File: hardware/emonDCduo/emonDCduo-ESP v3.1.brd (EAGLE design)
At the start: 99.1 x 76.5 mm, 73 parts, among them J5 455-1750-1-ND, P1 B4B-PH-K, Y1 32Khz

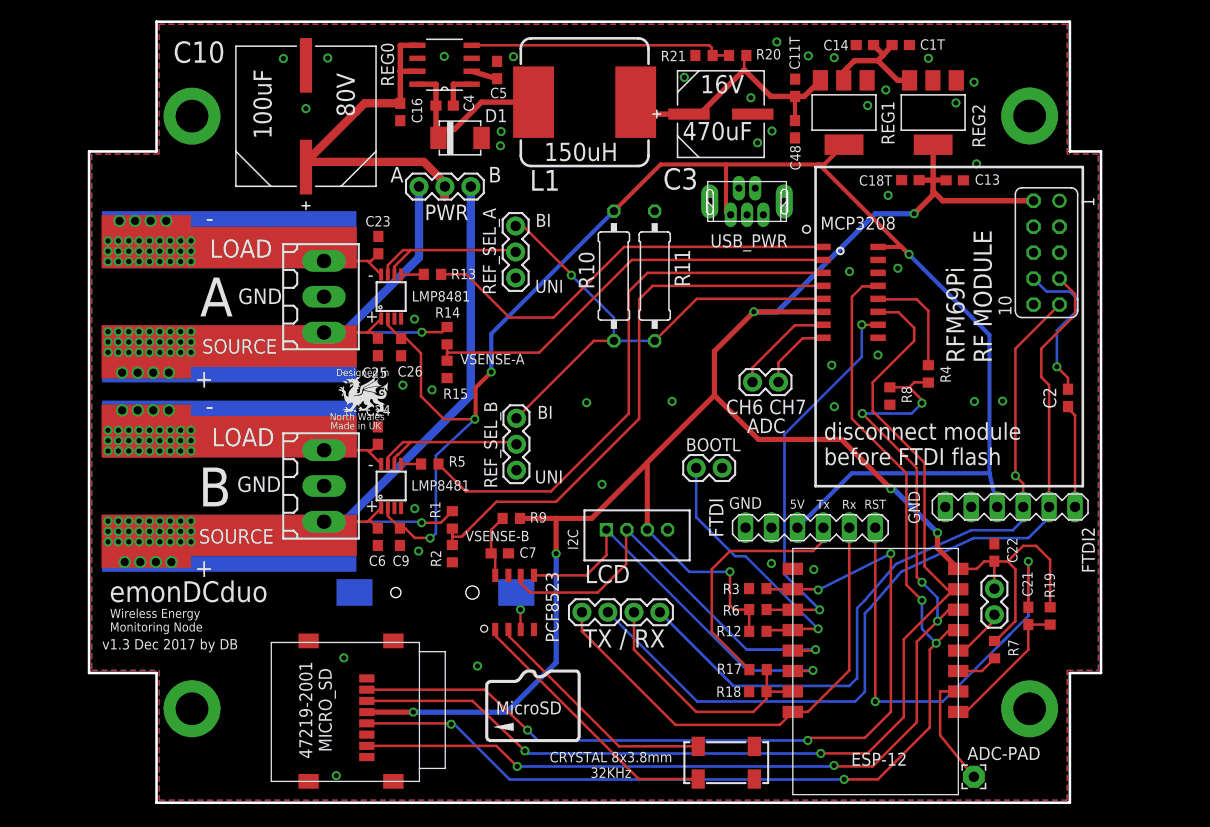
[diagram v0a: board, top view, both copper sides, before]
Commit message: commit v3.1
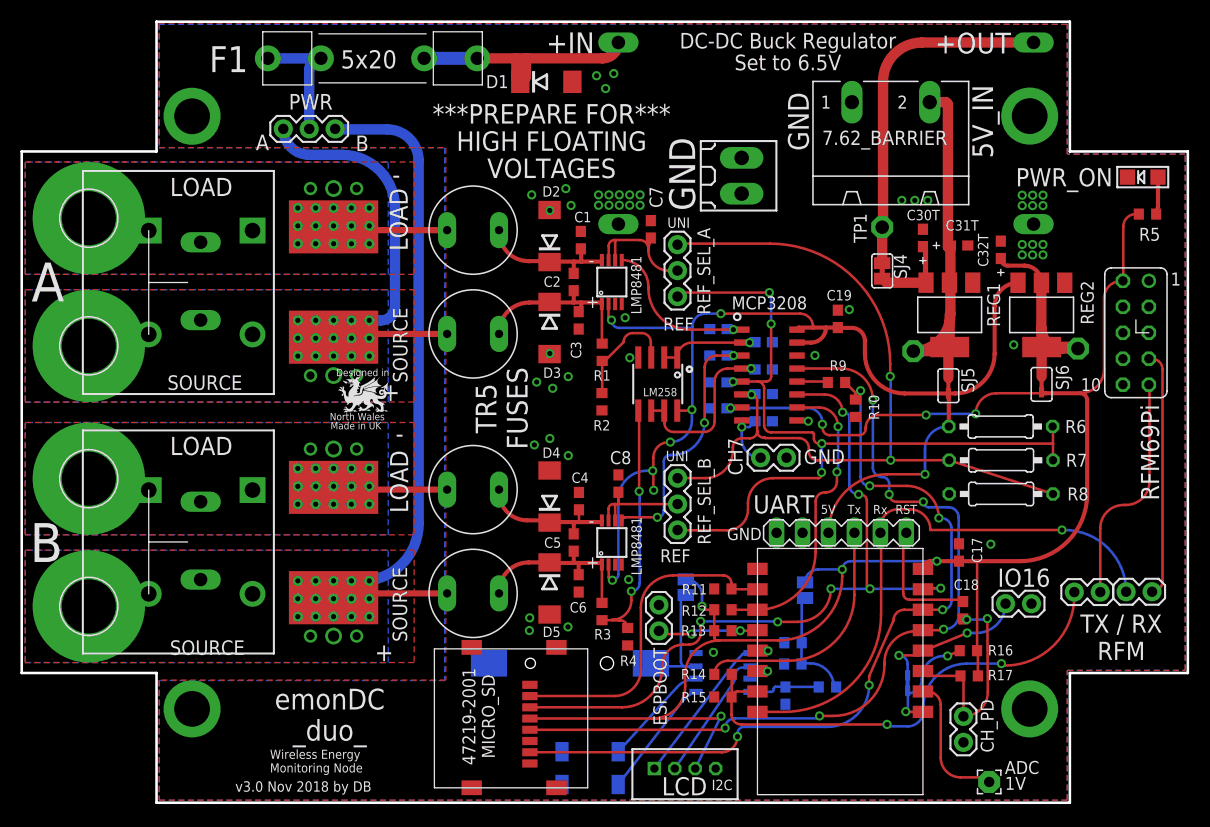
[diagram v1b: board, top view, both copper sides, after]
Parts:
- removed ADC-PAD: (no value), wirepad:2,15/1,0
- removed BOOTL, IO1: (no value), SparkFun:1X02
- removed C11T, C18T, C1T: 10uF TANT, rcl:C0603
- removed C21, C22, C26: 100nF, rcl:C0603
- removed C23, C24, C25: 0.1uF 100V, rcl:C0603
- removed C48: 0.1uF MLCC, rcl:C0603
- removed FTDI1, FTDI2: FTDI, JeeLabs:MA06-1
- removed L1: SRR1208, inductor-bourns:SSR1208
- removed R18, R19: 10K, rcl:R0603
- removed REG0: MAX5035, MAX5035:21-0111D_SBE-14
- removed SCREW1, SCREW2: (no value), con-weidmueller-sl35:180-3
- removed SCREW_TERM_1, SCREW_TERM_2: EBW_SERIES_15.2MM, EBW series shunt:EBW_SERIES_15.2MM
- removed U$4: 47219-2001_MICROSD, MOLEX 47219-2001:47219-2001_MICROSD
- removed USB_PWR: 5000751517_SD, 5000751517_sd:5000751517_SD
- added 3.3V_BAT, SJ4: (no value), jumper-con:SJ-CON
- added 7.62_BARRIER: GMSTBA2, con-phoenix-762:GMSTBA2
- added ADC: (no value), wirepad:2,15/1,0
- added C1, C8: 0.1uF 100V, rcl:C0603
- added C11, C12, C15: 1nF, rcl:C0603
- added C17, C18, C19: 0.1uF, rcl:C0603
- added C30T, C31T, C32T, C33T: 10uF TANT, rcl7:C0603POL
- added CH_PD, ESPBOOT: (no value), SparkFun:1X02
- added D2, D3, D4, D5: P6SMB75A, diode:DO214AA
- added EBW_A, EBW_B: EBW_SERIES_15.2MM, EBW series SHUNT:EBW_SERIES_15.2MM
- added F1: 445/030_SERIES, LITTELFUSE 455:030 SERIES:445/030_SERIES_LITTELFUSE
- added F2, F3, F4, F5: (no value), fuse:TR5
- added GND: (no value), con-weidmueller-sl35_db:180-2
- added IO16: FACTORY_RESET, SparkFun:1X02
- added LED1: PWR_ON, microbuilder:CHIPLED_1206
- added LM258: (no value), microbuilder:SOIC8_150MIL
- added MH1, MH2, MH3, MH4: 5.3mm, holes-db:5,3//11-PAD
- added MICRO_SD: 47219-2001_MICROSD, MOLEX 47219-2001:47219-2001_MICROSD
- added MOUNT_10.16_A, MOUNT_10.16_B: MOLEX_39970-003, 10.16mm terminal block:2/10,16
- added R16: 10K, rcl:R0603
- added R22: 1K, rcl@1:R0603
- added SJ1, SJ5, SJ6: (no value), jumper-con_db:SJ-CON
- added SJ2: (no value), jumper:SJ
- added TP1, TP2, TP3: TPPAD1-13, testpad:P1-13
- added TP10, TP11, TP4, TP5, TP6, TP7, TP8, TP9: TPPAD1-13Y, testpad:P1-13Y
- added U$2, U$3: (no value), ALIGNMENT_STOP:ALIGNMENT_STOP
- added UART: UART, JeeLabs:MA06-1
- C10: value 100uF 80V (LOW-ESR) -> 1nF; device Panasonic-EEE-EEV-EEF-ECQ:CAPAE1350X1400N -> rcl:C0603
- C13, C14: value 0.1uF -> 1nF
- C16: value 0.1uF 100V -> 1nF
- C2: value 100nF -> 0.1uF 100V
- C3: value 470uF 16V -> 0.1uF 100V; device Panasonic-EEEFK_EEEFP:CAPAE830X1050N -> rcl:C0603
- C4, C5: value 0.1uF 16V MLCC -> 0.1uF 100V
- C7: value 10uF -> 0.1uF 100V
- C9: value 100nF -> 1nF
- D1: value MBRS1100T3G -> P6SMB75A; device diodes:SMB_1 -> diode:DO214AA
- GPIO_1: device con-lsta:FE05-2 -> con-lsta-RFM69Pi:FE05-2_RFM69PI_OULTINE
- J5: value 455-1750-1-ND -> (none)
- P1: device jst-ph:B4B-PH-K -> JST-PH:B4B-PH-K
- PCF8523: device IotaWatt_parts:SOIC_8 -> emonDC parts:SOIC_8
- R1: value 100K 75V -> 1M 100V
- R10: value 10K -> 2K; device rcl:0309/12 -> rcl:R0603
- R11: value 3.16K -> 10K; device rcl:0309/12 -> rcl:R0603
- R13: value 1K -> 10K
- R14: value 100K 75V -> 1k
- R15: value 5.6K -> 2k
- R17: value 5.6K -> 10K
- R2: value 5.6K -> 56K
- R20: value 57.6k -> 10K
- R21: value 13.3k -> 10K
- R3: value 10K -> 1M 100V
- R4: value 1K -> 56K
- R5: value 1K -> 174R
- R6: value 10K -> 10k; device rcl:R0603 -> rcl7:0207/10
- R7: value 10K -> 5.6k; device rcl:R0603 -> rcl7:0207/10
- R8: value 2K -> 174R; device rcl:R0603 -> rcl7:0207/10
- REG1, REG2: device burr-brown:SOT223 -> burr-brown-db:SOT223
- moved R5 74.4 mm to (103.9, 59.4), turned to 180 degrees
- moved R21 60.2 mm to (69.1, 15.4), flipped to the bottom
- moved LOGO1 59.5 mm to (81.6, 2.56)
- moved R20 57.7 mm to (69.2, 17.4), flipped to the bottom
- moved TX 53.3 mm to (101.8, 22.4)
- moved C10 50.0 mm to (66.3, 46.9), flipped to the bottom, turned to 180 degrees
- moved C2 49.7 mm to (47.7, 52.8)
- moved C5 46.9 mm to (47.7, 27.2), turned to 270 degrees
- moved C16 46.7 mm to (66.3, 39.1), flipped to the bottom, turned to 180 degrees
- moved R13 45.0 mm to (62.3, 18.6), turned to 180 degrees
- moved RX 43.2 mm to (99.2, 22.4)
- moved R14 42.8 mm to (62.3, 14.3), turned to 0 degrees
- moved R15 41.9 mm to (62.3, 12.1), turned to 180 degrees
- moved C4 40.9 mm to (48.2, 31.3), turned to 90 degrees
- moved R4 39.1 mm to (53.0, 18.0)
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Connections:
- removed net 3.3V: C13.1, C18T.1, C22.2, ESP-12.16, GPIO_1.2, IO1.2, MCP3208.6, P1.3, R12.2, R19.2, R6.2, R7.2, R9.2, REG2.2, REG2.4, U$4.PIN4
- removed net 5.0V: C14.1, C1T.1, C26.1, C9.1, FTDI1.4, FTDI2.4, MCP3208.16, R10.2, REG1.2, REG1.4, REG2.3, SHUNTMON-A.2, SHUNTMON-B.2, USB_PWR.VBUS
- removed net ADCSHUNT-A: MCP3208.1, R13.2
- removed net ADCSHUNT-B: MCP3208.3, R5.2
- removed net BST: C4.1, REG0.1
- removed net CH6: J5.2, MCP3208.7
- removed net FB: R20.1, R21.2, REG0.4
- removed net LX: C4.2, D1.C, L1.1, REG0.8
- removed net N$10: C7.1, PCF8523.8, R9.1
- removed net N$20: FTDI2.5
- removed net N$30: C21.2, FTDI1.1
- removed net N$301: C2.2, FTDI2.1
- removed net N$4: R13.1, SHUNTMON-A.5
- removed net N$43: CR1220.P+, PCF8523.3
- removed net N$6: R5.1, SHUNTMON-B.5
- removed net REF_INPUT: MCP3208.5, R10.1, R11.2, REF_SEL_A.3, REF_SEL_B.3
- removed net RESTESP: C21.1, ESP-12.9, R19.1
- removed net VD: C5.1, REG0.2
- removed net VSENSEA: MCP3208.2, R14.1, R15.2
- removed net VSENSEB: MCP3208.4, R1.1, R2.2
- removed net V_IN: C10.1, C16.1, PWR.2, REG0.5, REG0.7
- new net +3V3: 3.3V_BAT.1, C15.1, C17.2, ESP-12.16, GPIO_1.2, MCP3208.7, MICRO_SD.PIN4, P1.3, R12.2, R13.2, R16.2, R17.2, R5.2, SJ2.1, SJ6.2
- new net +5V: C19.1, LM258.8, MCP3208.15, MCP3208.16, R6.2, REG2.3, SHUNTMON-A.2, SHUNTMON-B.2, SJ5.2, UART.4
- new net 3.3V_PRE: C32T.1, REG2.2, REG2.4, SJ6.1, TP3.TP
- new net 5V_PRE: 7.62_BARRIER.2, C31T.1, REG1.2, REG1.4, SJ5.1, TP2.TP
- new net ADCSHUNT_A: C9.1, MCP3208.1, SHUNTMON-A.5
- new net ADCSHUNT_B: C11.1, MCP3208.3, SHUNTMON-B.5
- new net BI_REF: C13.1, MCP3208.5, R6.1, R7.2, REF_SEL_A.3, REF_SEL_B.3
- new net LOAD-NEG-A_T: C1.1, C2.1, D2.C, F2.2, SHUNTMON-A.8
- new net LOAD-NEG-B_T: C4.1, C5.1, D4.C, F4.2, SHUNTMON-B.8
- new net N$1: SJ4.1, TP1.TP, TP5.TP
- new net N$5: LED1.A, R5.1
- new net RESET: C18.2, UART.1
- new net RST: ESP-12.9, R16.1, SJ1.1
- new net SOURCE-POS-A_T: C2.2, C3.1, D3.C, F3.2, R1.2, SHUNTMON-A.1
- new net SOURCE-POS-B_T: C5.2, C6.1, D5.C, F5.2, R3.2, SHUNTMON-B.1
- new net UNI_REF: C14.1, MCP3208.6, R7.1, R8.2, REF_SEL_A.1, REF_SEL_B.1
- new net VBAT: 3.3V_BAT.2, CR1220.P+, PCF8523.3
- new net VDD_PCF: C33T.1, PCF8523.8, R22.1
- new net VDD_RTC_POSTJUMPER: R20.1, R21.1, R22.2, SJ2.2
- new net VSENSE_A: LM258.3, R1.1, R2.2
- new net VSENSE_A_BUFF: C10.1, LM258.1, LM258.2, MCP3208.2
- new net VSENSE_B: LM258.5, R3.1, R4.2
- new net VSENSE_B_BUFF: C12.1, LM258.6, LM258.7, MCP3208.4
- new net V_IN_POSTFUSE: D1.C, F1.P$3, F1.P$4, TP4.TP
- new net V_IN_PREFUSE: F1.P$1, F1.P$2, PWR.2
- net 6.5V: now also C30T.1, SJ4.2; no longer C11T.1, C3.1, C48.1, L1.2, R20.2
- net ADC: now also ADC.1; no longer ADC-PAD.1
- net CH7: now also C16.1
- net CH_PD: now also C18.1, CH_PD.1, R17.1; no longer R7.1
- net D0/RX: no longer FTDI2.2
- net D1/TX: no longer FTDI2.3
- net ESPRX: now also R14.2, R15.1; no longer R17.2, R18.1
- net ESPTX: now also UART.2; no longer FTDI1.2
- net GND: now also 7.62_BARRIER.1, C1.2, C17.1, C19.2, C30T.2, C31T.2, C32T.2, C33T.2, C4.2, C8.2, CH_PD.2, D2.A, D3.A, D4.A, D5.A, ESPBOOT.1, GND.1, GND.2, IO16.2, J5.2, LED1.C, LM258.4, MICRO_SD.P$1, MICRO_SD.P$2, MICRO_SD.P$3, MICRO_SD.P$4, MICRO_SD.PIN6, R10.2, R11.2, R15.2, R4.1, TP6.TP, TP7.TP, UART.6; no longer BOOTL.1, C10.2, C11T.2, C13.2, C14.2, C16.2, C18T.2, C1T.2, C22.1, C23.1, C24.1, C25.2, C26.2, C48.2, C5.2, C9.2, FTDI1.6, FTDI2.6, MCP3208.15, R11.1, R15.1, R18.2, R21.1, R3.2, REF_SEL_A.1, REF_SEL_B.1, REG0.3, REG0.6, SCREW1.2, SCREW2.2, U$4.P$1, U$4.P$2, U$4.P$3, U$4.P$4, U$4.PIN6, USB_PWR.GND1, USB_PWR.GND2, USB_PWR.GND3
- net GPIO0: now also ESPBOOT.2, R13.1; no longer BOOTL.2, R12.1
- net GPIO12: now also MICRO_SD.PIN7, R10.1, R9.2; no longer R4.1, R8.2, U$4.PIN7
- net GPIO12A: now also R9.1; no longer R4.2
- net GPIO13: now also MICRO_SD.PIN3; no longer U$4.PIN3
- net GPIO14: now also MICRO_SD.PIN5; no longer U$4.PIN5
- net GPIO15: now also MICRO_SD.PIN2, R11.1; no longer R3.1, U$4.PIN2
- net GPIO16: now also IO16.1, SJ1.2; no longer IO1.1
- net GPIO2: now also R12.1; no longer R6.1
- net LOAD-NEG-A: now also EBW_B.P$18, EBW_B.P$19, EBW_B.P$2, EBW_B.P$20, EBW_B.P$21, EBW_B.P$22, EBW_B.P$23, EBW_B.P$24, EBW_B.P$25, EBW_B.P$26, EBW_B.P$27, EBW_B.P$28, EBW_B.P$29, EBW_B.P$30, EBW_B.P$31, EBW_B.P$32, EBW_B.P$36, EBW_B.P$37, EBW_B.P$38, F2.1, MH2.B5,5, MOUNT_10.16_A.P$1, MOUNT_10.16_A.P$2, TP11.TP; no longer C23.2, SCREW1.1, SCREW_TERM_1.P$2, SHUNTMON-A.8
- net LOAD-NEG-B: now also EBW_A.P$18, EBW_A.P$19, EBW_A.P$2, EBW_A.P$20, EBW_A.P$21, EBW_A.P$22, EBW_A.P$23, EBW_A.P$24, EBW_A.P$25, EBW_A.P$26, EBW_A.P$27, EBW_A.P$28, EBW_A.P$29, EBW_A.P$30, EBW_A.P$31, EBW_A.P$32, EBW_A.P$36, EBW_A.P$37, EBW_A.P$38, F4.1, MH4.B5,5, MOUNT_10.16_B.P$1, MOUNT_10.16_B.P$2, TP9.TP; no longer C24.2, SCREW2.1, SCREW_TERM_2.P$2, SHUNTMON-B.8
- net N$32: now also MICRO_SD.PIN8; no longer U$4.PIN8
- net N$36: now also R14.1, UART.3; no longer FTDI1.3, R17.1
- net N$7: now also MICRO_SD.PIN1; no longer U$4.PIN1
- net REF_A_INPUT: now also C7.1
- net REF_B_INPUT: now also C8.1
- net SCL: now also ESP-12.6; no longer ESP-12.5
- net SDA: now also ESP-12.5; no longer ESP-12.6
- net SOURCE-POS-A: now also EBW_B.P$1, EBW_B.P$10, EBW_B.P$11, EBW_B.P$12, EBW_B.P$13, EBW_B.P$14, EBW_B.P$15, EBW_B.P$16, EBW_B.P$17, EBW_B.P$3, EBW_B.P$33, EBW_B.P$34, EBW_B.P$35, EBW_B.P$4, EBW_B.P$5, EBW_B.P$6, EBW_B.P$7, EBW_B.P$8, EBW_B.P$9, F3.1, MH1.B5,5, MOUNT_10.16_A.P$3, MOUNT_10.16_A.P$4, TP10.TP; no longer C25.1, R14.2, SCREW1.3, SCREW_TERM_1.P$1, SHUNTMON-A.1
- net SOURCE-POS-B: now also EBW_A.P$1, EBW_A.P$10, EBW_A.P$11, EBW_A.P$12, EBW_A.P$13, EBW_A.P$14, EBW_A.P$15, EBW_A.P$16, EBW_A.P$17, EBW_A.P$3, EBW_A.P$33, EBW_A.P$34, EBW_A.P$35, EBW_A.P$4, EBW_A.P$5, EBW_A.P$6, EBW_A.P$7, EBW_A.P$8, EBW_A.P$9, F5.1, MH3.B5,5, MOUNT_10.16_B.P$3, MOUNT_10.16_B.P$4, TP8.TP; no longer C6.1, R1.2, SCREW2.3, SCREW_TERM_2.P$1, SHUNTMON-B.1
- net _RESET: no longer C2.1
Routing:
- net 3.3V: track 198.0 -> 0.00 mm, vias 7 -> 0
- net +3V3: track 0.00 -> 172.3 mm, vias 0 -> 8
- net 5.0V: track 171.2 -> 0.00 mm, vias 4 -> 0
- net +5V: track 0.00 -> 113.2 mm, vias 0 -> 8
- net UNI_REF: track 0.00 -> 81.1 mm, vias 0 -> 3
- net BI_REF: track 0.00 -> 79.0 mm, vias 0 -> 5
- net D0/RX: track 84.0 -> 24.0 mm
- net VSENSEB: track 55.7 -> 0.00 mm
- net ADCSHUNT-B: track 54.6 -> 0.00 mm
- net 5V_PRE: track 0.00 -> 53.8 mm
- net GPIO15: track 83.0 -> 31.6 mm, vias 4 -> 0
- net REF_INPUT: track 50.5 -> 0.00 mm, vias 1 -> 0
- net D1/TX: track 72.0 -> 22.5 mm, vias 1 -> 0
- net N$30: track 47.1 -> 0.00 mm, vias 2 -> 0
- net VSENSEA: track 42.3 -> 0.00 mm
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- added copper zone on layer 1, net LOAD-NEG-A
- added copper zone on layer 16, net LOAD-NEG-A
- added copper zone on layer 1, net LOAD-NEG-B
- added copper zone on layer 16, net LOAD-NEG-B
- added copper zone on layer 1, net SOURCE-POS-A
- added copper zone on layer 16, net SOURCE-POS-A
- added copper zone on layer 1, net SOURCE-POS-B
- added copper zone on layer 16, net SOURCE-POS-B
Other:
- board size 99.1 x 76.5 mm -> 114.2 x 76.5 mm
- board text added: "***PREPARE FOR*** HIGH FLOATING VOLTAGES"
- board text added: "+IN"
- board text added: "+OUT"
- board text added: "1V"
- board text added: "5V_IN"
- board text added: "5x20"
- board text added: "CH7"
- board text added: "DC-DC Buck Regulator Set to 6.5V"
- board text added: "Designed in North Wales"
- board text added: "Open Hardware"
- board text added: "PWR_ON"
- board text added: "REF"
- board text added: "RFM69Pi"
- board text added: "TR5 FUSES"
- board text added: "TX / RX RFM"
- board text added: "emonDC _duo_"
- board text added: "v3.0 Nov 2018 by DB"
- board text removed: "100uF"
- board text removed: "150uH"
- board text removed: "16V"
- board text removed: "470uF"
- board text removed: "80V"
- board text removed: "BI"
- board text removed: "CH6 CH7 ADC"
- board text removed: "CRYSTAL 8x3.8mm 32KHz"
- board text removed: "Format MicroSD card to FAT32. Place blank 'datalog.txt' file there."
- board text removed: "MicroSD"
- board text removed: "Node:"
- board text removed: "Open-Hardware"
- board text removed: "RFM69Pi RF MODULE"
- board text removed: "TX / RX"
- board text removed: "USB_PWR"
- board text removed: "VSENSE-A"
- board text removed: "VSENSE-B"
- board text removed: "disconnect module before FTDI flash"
- board text removed: "emonDCduo"
- board text removed: "v1.3 Dec 2017 by DB"
